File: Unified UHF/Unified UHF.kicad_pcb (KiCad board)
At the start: 2 copper layers, 82.5 x 82.5 mm, 82 parts, among them IC1 QPC1022SR, IC2 GRF5504, IC3 LHA-13LN+, IC4 QPC1022SR, J1 Conn_01x05, J2 Conn_01x02, J3 Conn_01x02, J4 Conn_01x01, J5 PCB.SMAFST.2H.A.HT, U1 AT86RF215-ZU, U2 NCS-62+, X1 TYETACSANF-26.000000

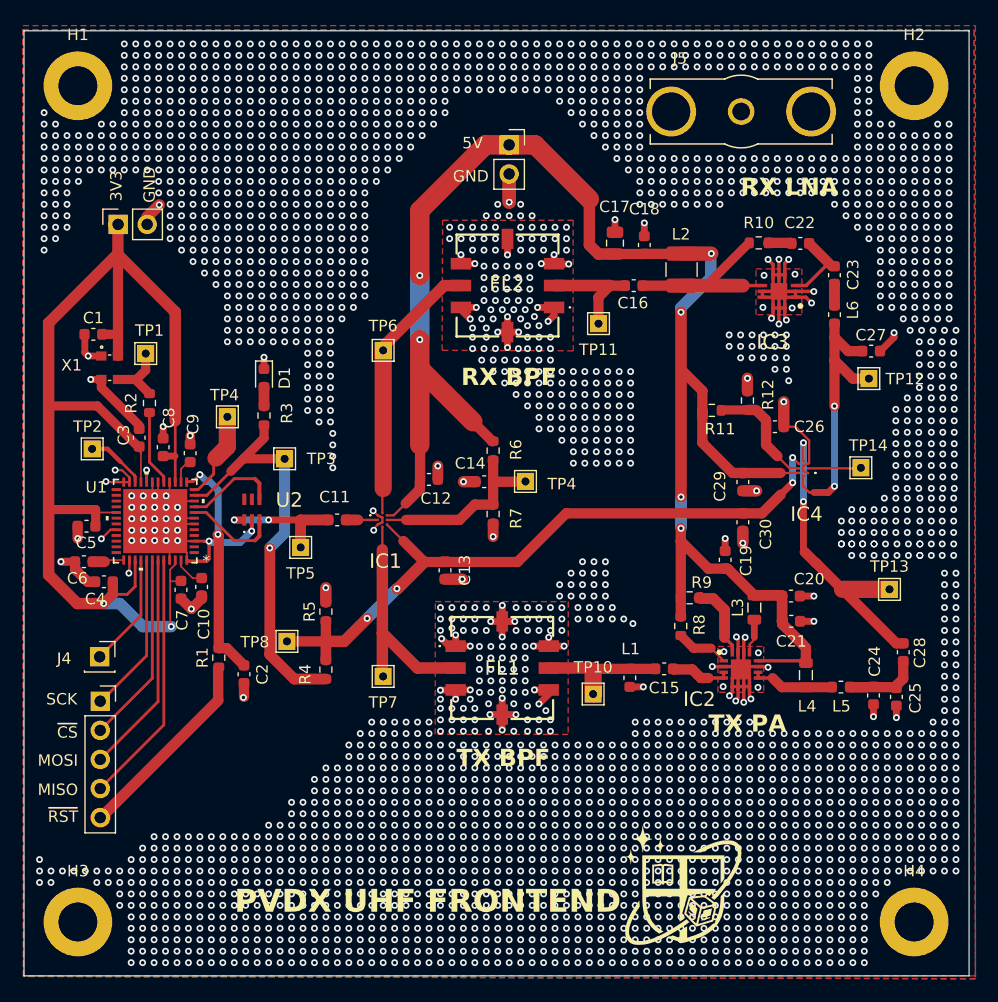
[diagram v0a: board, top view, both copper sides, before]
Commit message: Routed coax
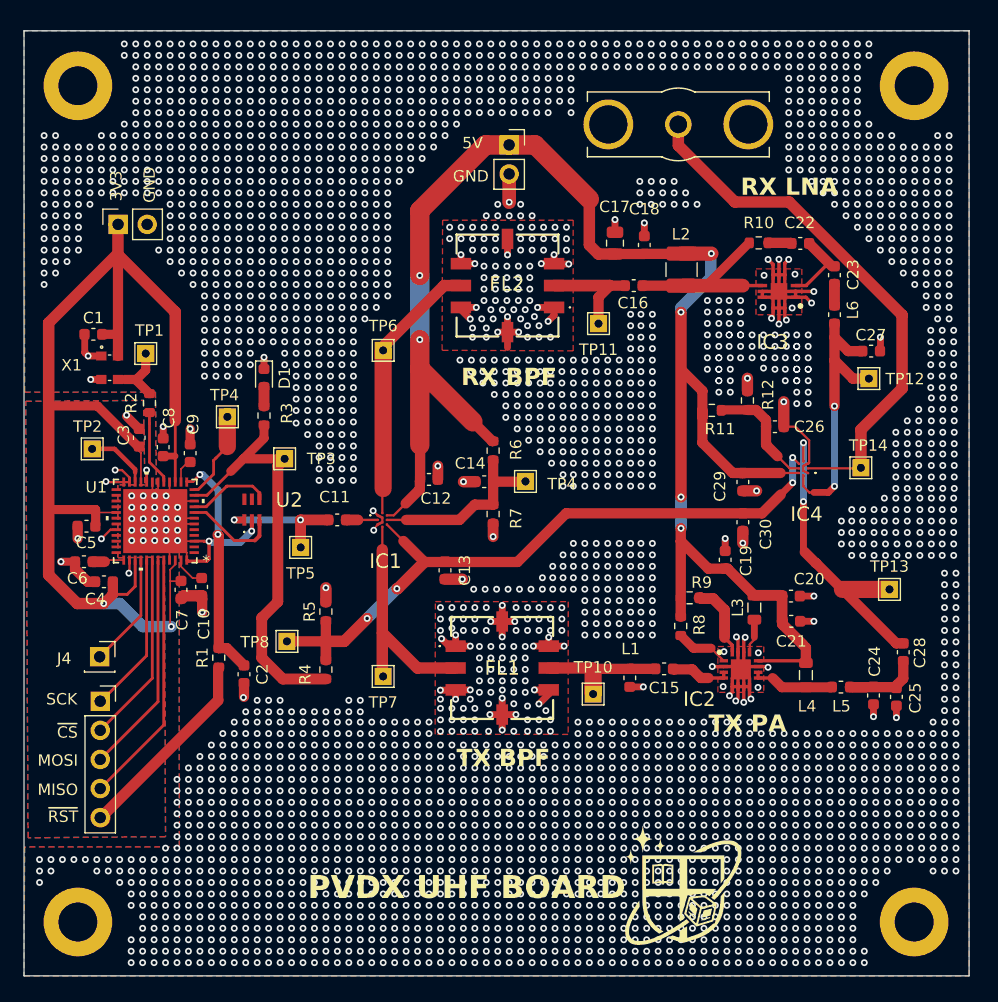
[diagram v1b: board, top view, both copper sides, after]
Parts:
- moved J5 5.60 mm to (88.0, 26.2)
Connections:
- C3 pad 1: GND -> GNDD
- C4 pad 1: GND -> GNDD
- C5 pad 1: GND -> GNDD
- C6 pad 1: GND -> GNDD
- U1 pad 20: GND -> GNDD
- U1 pad 23: GND -> GNDD
- U1 pad 24: GND -> GNDD
- U1 pad 32: GND -> GNDD
- U1 pad 38: GND -> GNDD
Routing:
- net Net-(IC4-ANT): track 4.63 -> 46.9 mm
- net GND: track 189.3 -> 162.8 mm, vias 2977 -> 3321
- net GNDD: track 0.00 -> 14.5 mm, vias 0 -> 8
- net Net-(U1-RFN09): track 8.53 -> 7.21 mm
- net Net-(U1-FEA09): track 36.3 -> 37.4 mm, vias 1 -> 0
- added copper zone on B.Cu, net GNDD
- added copper zone on F.Cu, net GNDD
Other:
- board text added: "PVDX UHF BOARD"
- board text removed: "PVDX UHF FRONTEND"

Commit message: adjustments
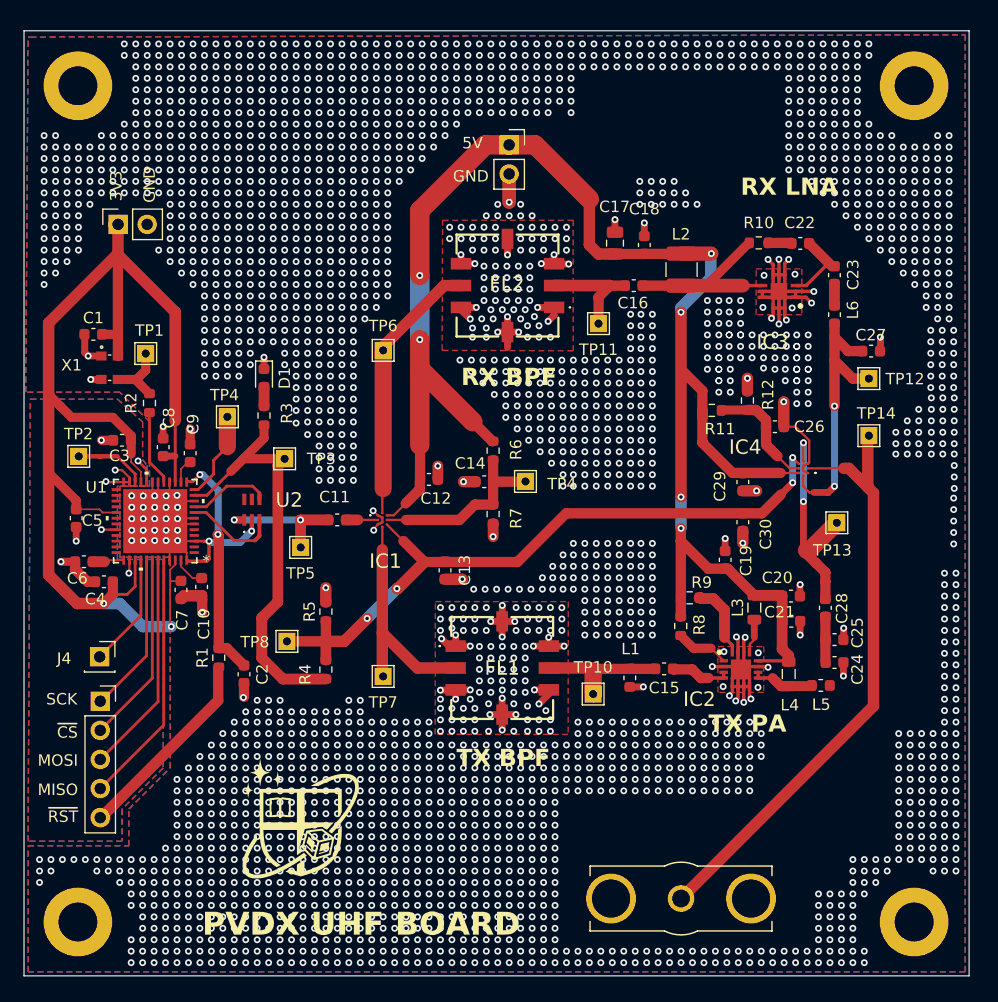
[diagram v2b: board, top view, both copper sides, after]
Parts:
- moved J5 67.6 mm to (88.2, 93.8)
- moved G*** 33.9 mm to (55.0, 87.2)
- moved C28 7.83 mm to (100.8, 68.4)
- moved TP13 7.41 mm to (101.8, 61.0)
- moved C25 7.36 mm to (101.6, 71.2), turned to 0 degrees
- moved C24 4.45 mm to (101.6, 73.2), turned to 0 degrees
- moved TP14 2.89 mm to (104.6, 53.4)
- moved L5 1.77 mm to (100.4, 75.2)
- moved C3 1.52 mm to (39.4, 53.8), turned to 0 degrees
- moved L4 1.50 mm to (97.6, 74.2)
- moved TP2 1.34 mm to (35.6, 55.2)
- moved C5 1.14 mm to (35.4, 60.6), turned to 90 degrees
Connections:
- H1 pad 1: (no net) -> GND
- H2 pad 1: (no net) -> GND
- H3 pad 1: (no net) -> GND
- H4 pad 1: (no net) -> GND
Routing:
- net Net-(IC4-RF1): track 27.2 -> 19.7 mm
- net Net-(IC4-ANT): track 46.9 -> 53.5 mm
- net Net-(C24-Pad1): track 7.76 -> 4.06 mm
- net +5V: track 143.1 -> 141.6 mm
- net +3V3: track 112.0 -> 113.2 mm
- net Net-(IC2-RF_OUT/VCC2_1): track 7.26 -> 6.18 mm
- net Net-(U1-CLKO): track 5.56 -> 6.41 mm
- net GND: track 162.8 -> 162.6 mm, vias 3321 -> 2852
- removed copper zone on B.Cu, net GNDD
- removed copper zone on F.Cu, net GNDD
